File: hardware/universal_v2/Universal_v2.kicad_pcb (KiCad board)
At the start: 2 copper layers, 15 parts, among them J1 DS18B20, J2 DEV_PORT, J4 Ext, P1 TC2030-CTX, U1 HolyIot-18010, U2 BME680, U3 SHT30-DIS-B

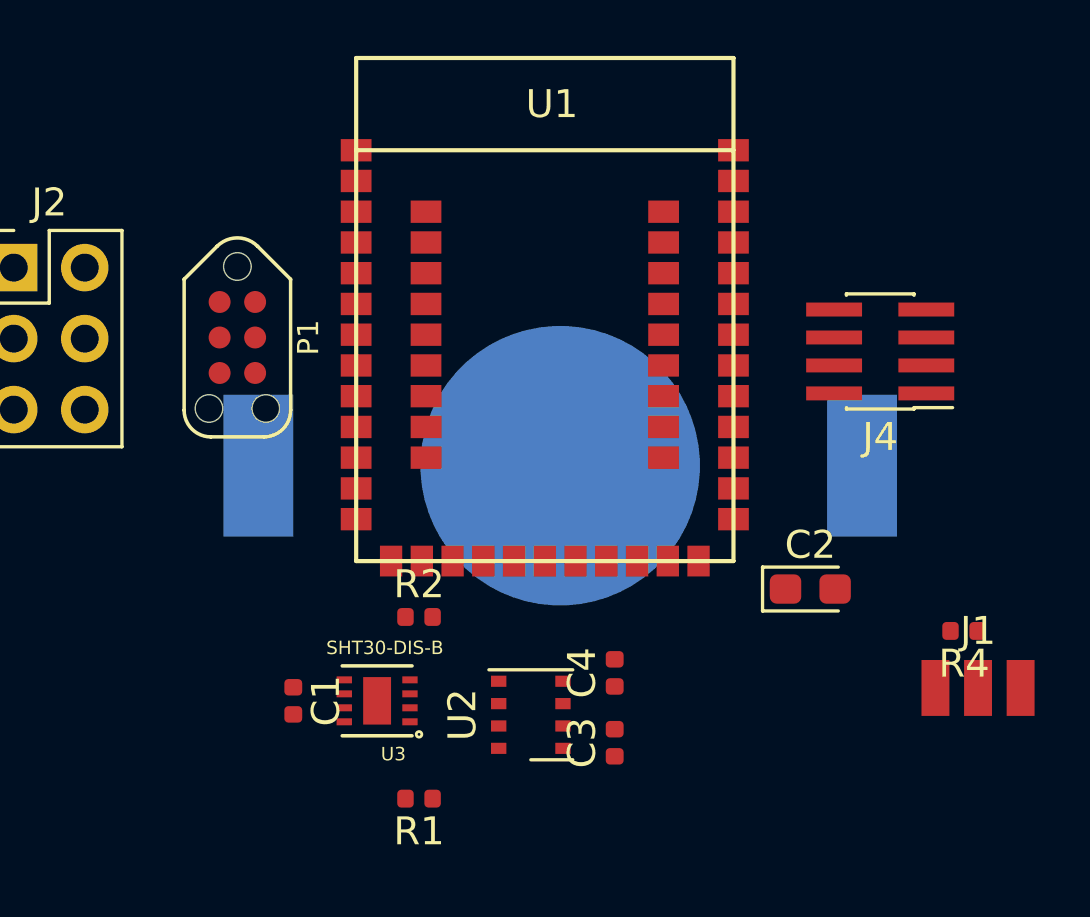
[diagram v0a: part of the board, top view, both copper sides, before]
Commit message: Another version of hardware concept
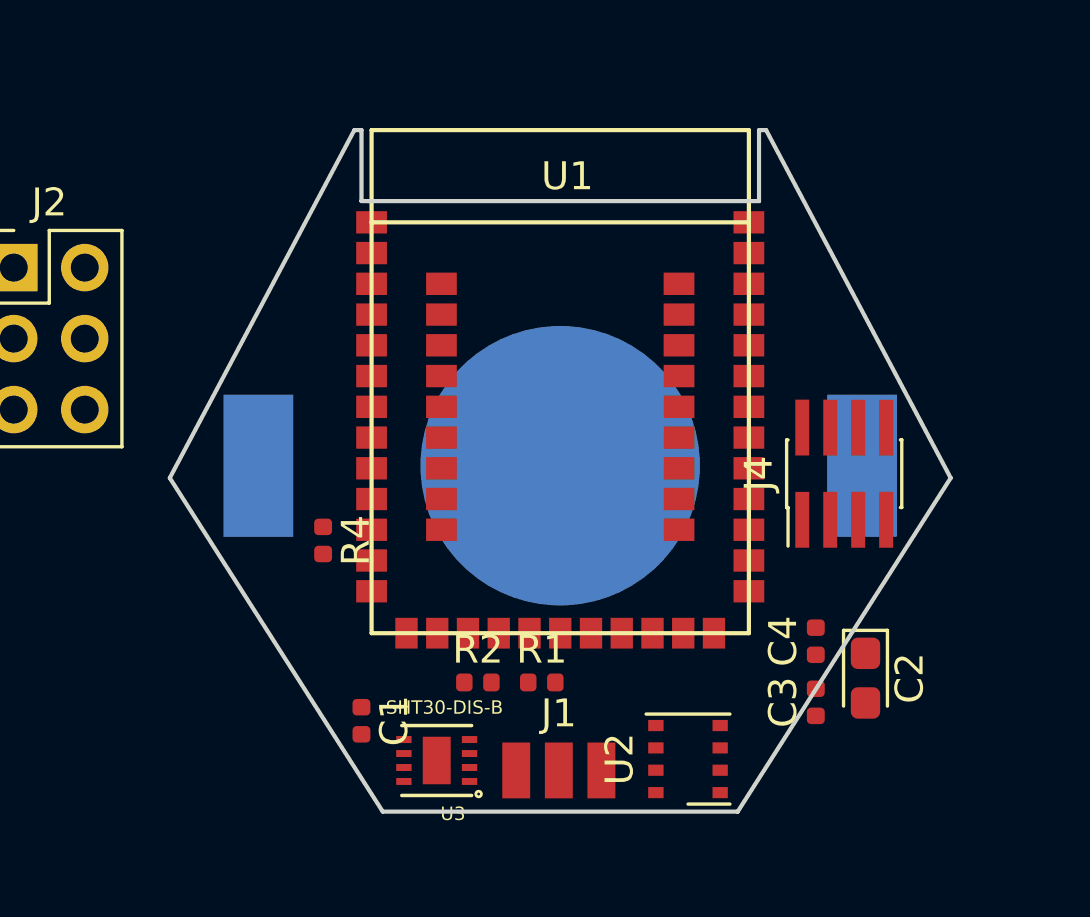
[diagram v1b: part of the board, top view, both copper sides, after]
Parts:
- removed P1: TC2030-CTX, Tag-Connect:TC2030-NL_SMALL
- moved R4 23.2 mm to (90.1, 83.3), turned to 270 degrees
- moved J1 15.3 mm to (98.5, 89.0)
- moved C3 7.34 mm to (107.7, 89.1)
- moved C4 7.28 mm to (107.7, 86.9)
- moved R1 6.05 mm to (97.9, 88.3), turned to 0 degrees
- moved U2 5.84 mm to (103.1, 91.1)
- moved J4 4.56 mm to (108.7, 80.9), turned to 90 degrees
- moved C2 3.75 mm to (109.5, 88.2), turned to 270 degrees
- moved R2 3.15 mm to (95.6, 88.3)
- moved U3 3.02 mm to (94.1, 91.1)
- moved U1 2.64 mm to (98.6, 68.6)
- moved C1 2.54 mm to (91.4, 89.7)
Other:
- board outline added: 27.9 x 24.4 mm

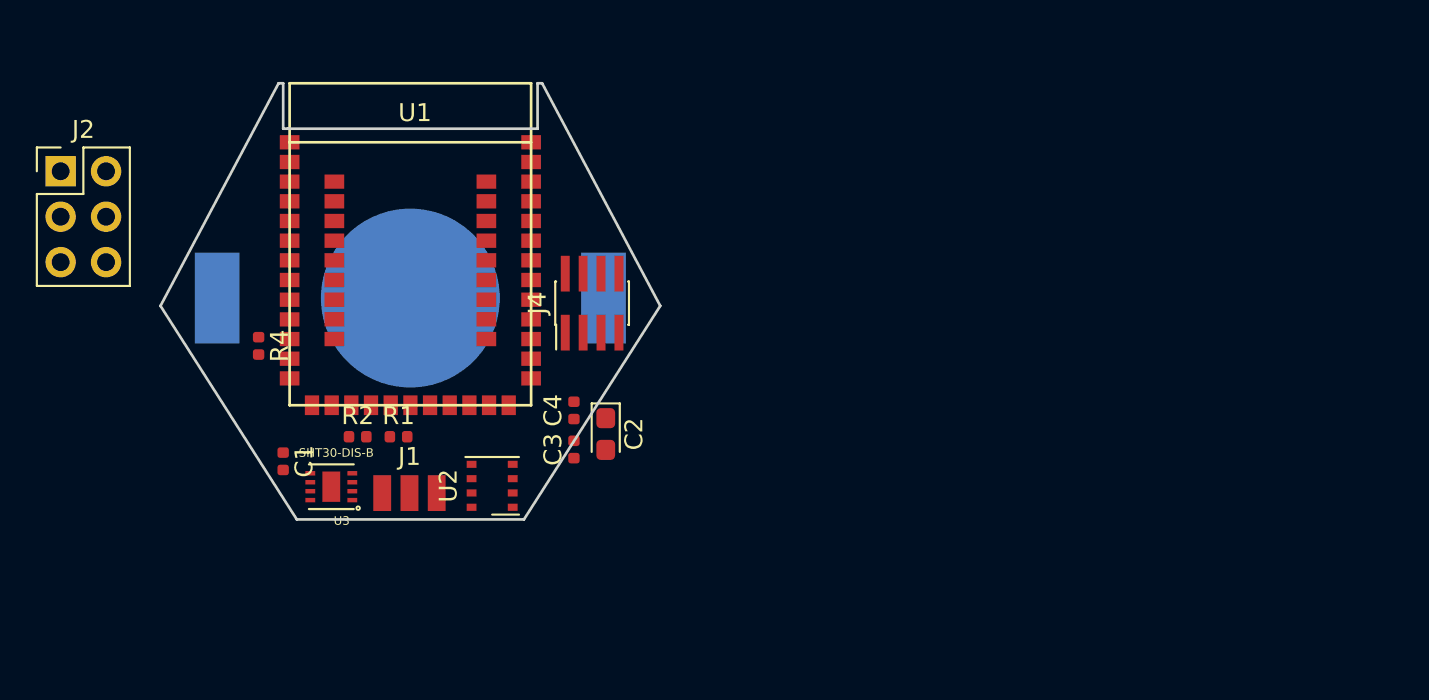
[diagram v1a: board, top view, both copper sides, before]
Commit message: Hardware v2, upgrade
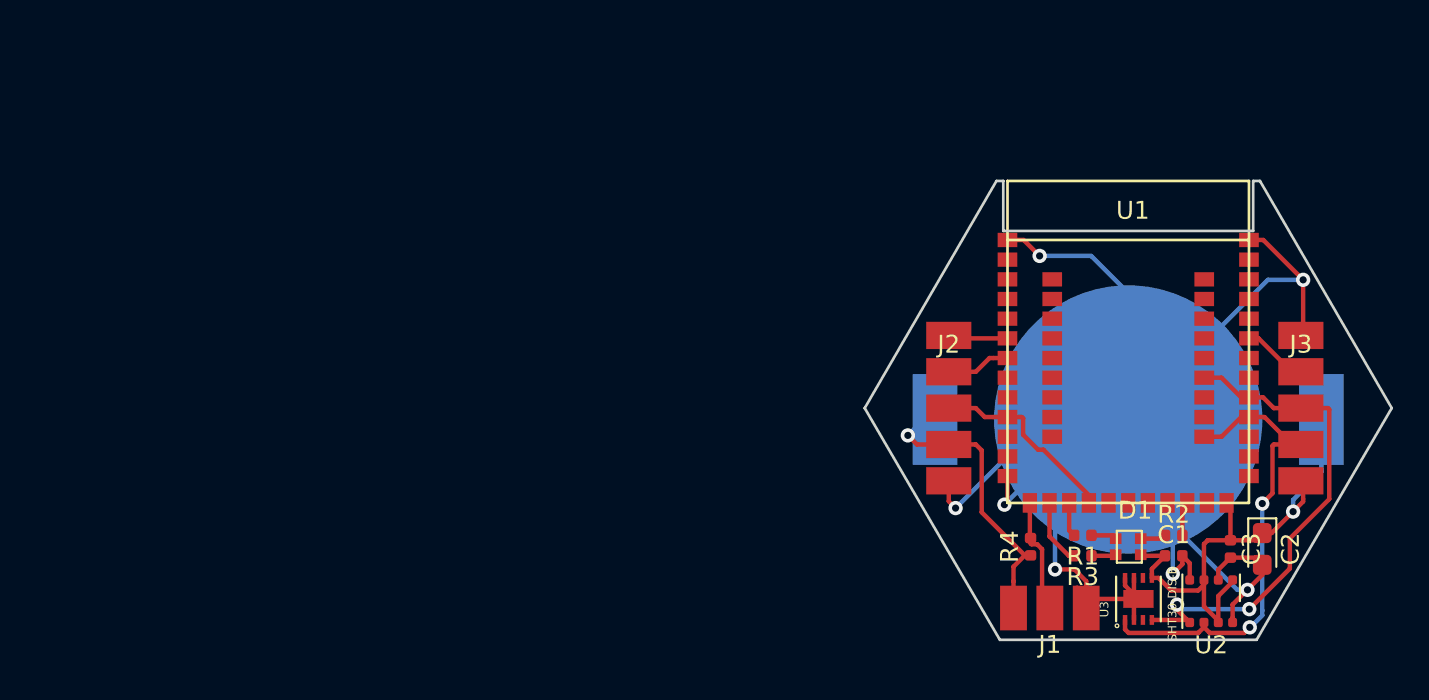
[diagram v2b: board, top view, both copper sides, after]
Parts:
- removed C4: 100nF, Capacitor_SMD:C_0402_1005Metric
- removed J4: Ext, Connector_PinHeader_1.00mm:PinHeader_2x04_P1.00mm_Vertical_SMD
- added D1: LED_BARG, Everlight:Everlight_19-237_R6GHBHC-M07_2T, F.Cu at (138.7, 94.5)
- added J3: EXT_PORT, Pads:5xPad, F.Cu at (148.3, 82.7)
- added R3: 10, Resistor_SMD:R_0402_1005Metric, F.Cu at (136.1, 95.0)
- J2: value DEV_PORT -> PROG_PORT; footprint Connector_PinHeader_2.54mm:PinHeader_2x03_P2.54mm_Vertical -> Pads:5xPad
- R1, R2: value 4,7k -> 10
- moved J2 50.5 mm to (128.7, 82.7)
- moved C1 50.1 mm to (141.2, 95.0), turned to 0 degrees
- moved R2 46.0 mm to (141.2, 93.9)
- moved U3 45.6 mm to (139.3, 97.4), turned to 90 degrees
- moved R4 44.6 mm to (133.2, 94.5), turned to 90 degrees
- moved U2 40.7 mm to (143.3, 97.5), turned to 180 degrees
- moved B1 40.7 mm to (138.7, 87.4)
- moved U1 40.5 mm to (138.7, 74.0)
- moved R1 38.6 mm to (136.1, 93.9), turned to 180 degrees
- moved J1 37.6 mm to (134.3, 100.5), turned to 180 degrees
- moved C2 37.3 mm to (146.2, 94.6)
- moved C3 37.1 mm to (144.4, 94.6), turned to 270 degrees
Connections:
- J1 pad 1: /DS18B20 -> GND
- J1 pad 2: +3V3 -> /DS18B20
- J1 pad 3: GND -> +3V3
- J2 pad 3: Net-(J2-Pad3) -> /nRESET
- J2 pad 5: /nRESET -> GND
- R1 pad 1: +3V3 -> Net-(D1-Pad3)
- R1 pad 2: /SDA -> /LED_R
- R2 pad 1: +3V3 -> Net-(D1-Pad4)
- R2 pad 2: /SCL -> /LED_G
- U1 pad 10: Net-(U1-Pad10) -> /SDA
- U1 pad 13: /DS18B20 -> Net-(U1-Pad13)
- U1 pad 41: Net-(U1-Pad41) -> /nRESET
- U1 pad 45: Net-(U1-Pad45) -> /DS18B20
- U1 pad 46: Net-(U1-Pad46) -> /LED_B
- U1 pad 47: Net-(U1-Pad47) -> /LED_R
- U1 pad 53: Net-(U1-Pad53) -> /LED_G
- U1 pad 6: /ANALOG-2 -> /ANALOG-1
- U1 pad 7: /ANALOG-1 -> Net-(U1-Pad7)
- U1 pad 8: /IO-1 -> Net-(U1-Pad8)
- U1 pad 9: /IO-2 -> /SCL
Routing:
- net GND: track 0.00 -> 113.9 mm, vias 0 -> 7
- net +3V3: track 0.00 -> 46.4 mm, vias 0 -> 2
- net /SCL: track 0.00 -> 28.3 mm, vias 0 -> 2
- net /SDA: track 0.00 -> 28.1 mm, vias 0 -> 2
- net /nRESET: track 0.00 -> 10.8 mm
- net /DS18B20: track 0.00 -> 6.52 mm
- net /ANALOG-1: track 0.00 -> 4.18 mm
- net /LED_B: track 0.00 -> 3.70 mm
- net /SWDCLK_EXT: track 0.00 -> 3.60 mm
- net /SWDIO_EXT: track 0.00 -> 3.35 mm
- net /LED_R: track 0.00 -> 1.93 mm
- net /LED_G: track 0.00 -> 1.93 mm
- net Net-(D1-Pad4): track 0.00 -> 1.43 mm
- net Net-(D1-Pad3): track 0.00 -> 1.43 mm
- net Net-(D1-Pad1): track 0.00 -> 1.38 mm
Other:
- board size 27.9 x 24.4 mm -> 29.5 x 25.7 mm
